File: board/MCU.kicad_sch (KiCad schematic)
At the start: 21 parts, among them Q1 NMOS, U1 1EDL8011XUMA1, U7 ESP32-S2-DEVKITM-1U

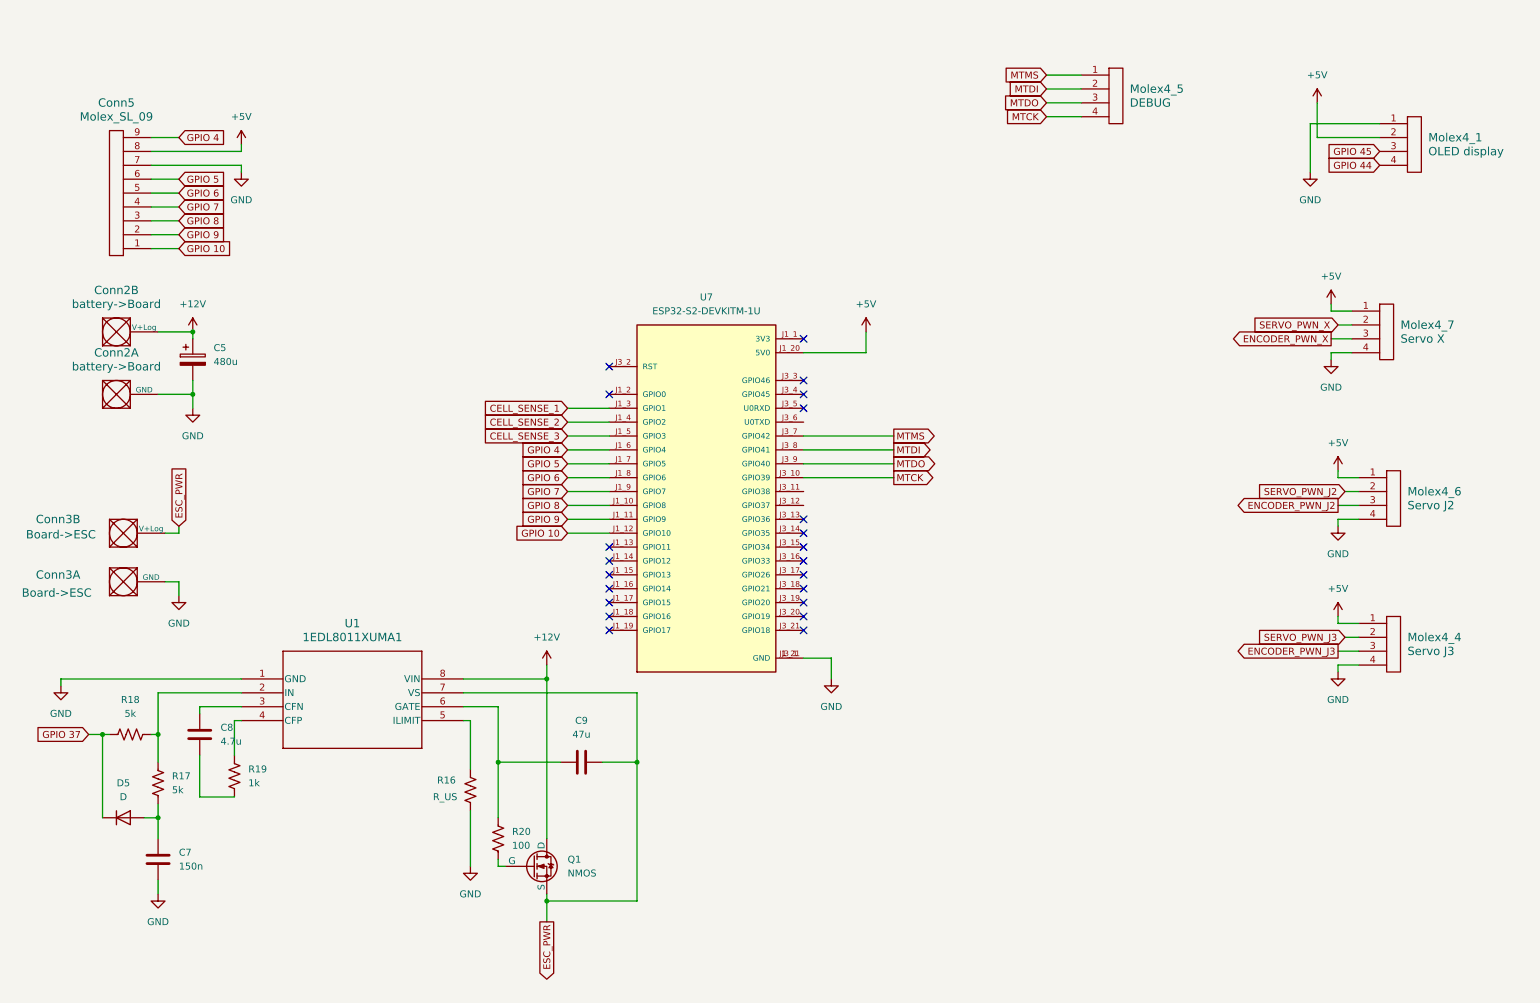
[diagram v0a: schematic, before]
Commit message: fixed some review issues and footprints
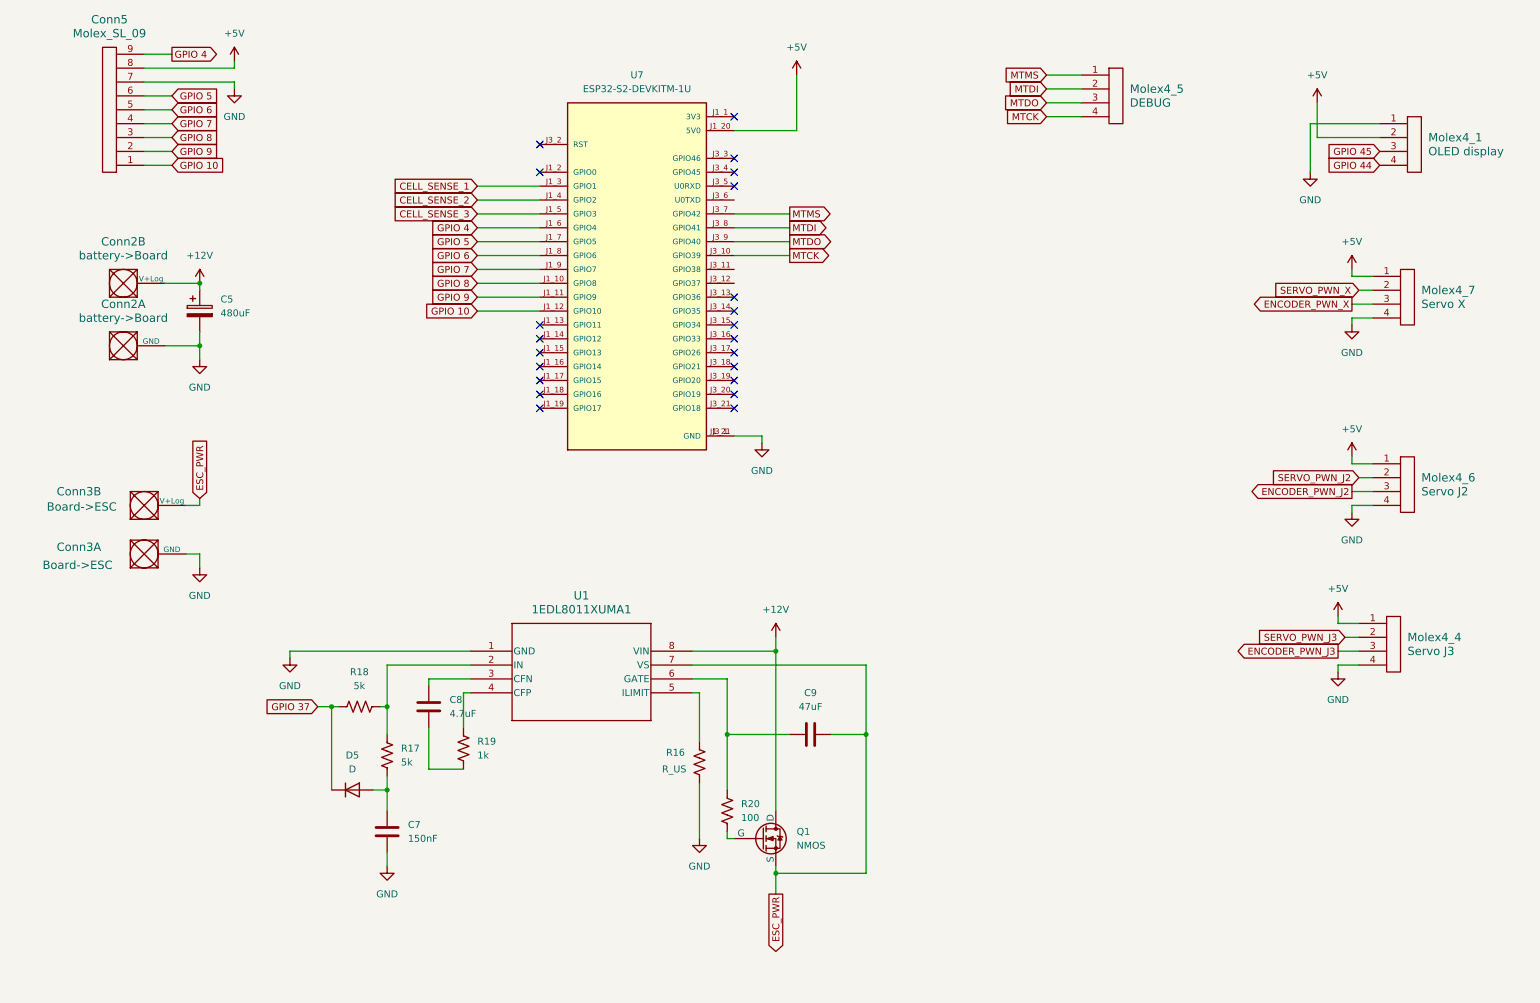
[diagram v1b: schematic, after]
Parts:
- C5: value 480u -> 480uF; footprint (none) -> Capacitor_SMD:C_0603_1608Metric_Pad1.08x0.95mm_HandSolder
- C7: value 150n -> 150nF; footprint (none) -> Capacitor_SMD:C_0603_1608Metric_Pad1.08x0.95mm_HandSolder
- C8: value 4.7u -> 4.7uF; footprint (none) -> Capacitor_SMD:C_0603_1608Metric_Pad1.08x0.95mm_HandSolder
- C9: value 47u -> 47uF; footprint (none) -> Capacitor_SMD:C_0603_1608Metric_Pad1.08x0.95mm_HandSolder
- Conn2, Conn3: footprint (none) -> MRDT_Connectors:Anderson_2_Horizontal_Side_by_Side
- Conn5, Molex4_1, Molex4_4, Molex4_5, Molex4_6, Molex4_7: footprint (none) -> MRDT_Connectors:MOLEX_SL_04_Vertical
- D5: footprint (none) -> Diode_SMD:D_0603_1608Metric
- R16, R17, R18, R19, R20: footprint (none) -> Resistor_SMD:R_0603_1608Metric_Pad0.98x0.95mm_HandSolder
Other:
- moved on the sheet: C5, C7, C8, C9, Conn2A, Conn2B, Conn3A, Conn3B, Conn5, D5, Molex4_6, Molex4_7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
